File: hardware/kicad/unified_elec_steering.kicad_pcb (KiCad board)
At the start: 2 copper layers, 77.2 x 87.7 mm, 24 parts, among them J1 Conn_01x03, J10 Conn_01x04, J11 Conn_01x03, J13 Conn_01x03, J2 Conn_01x03, J3 Conn_01x05, J4 Conn_01x03, J5 Conn_01x03, J6 Conn_01x02, J7 Conn_01x04, J8 Conn_01x12, J9 Conn_01x04, U1 Arduino_Nano_v3.x, U2 D24V150F7

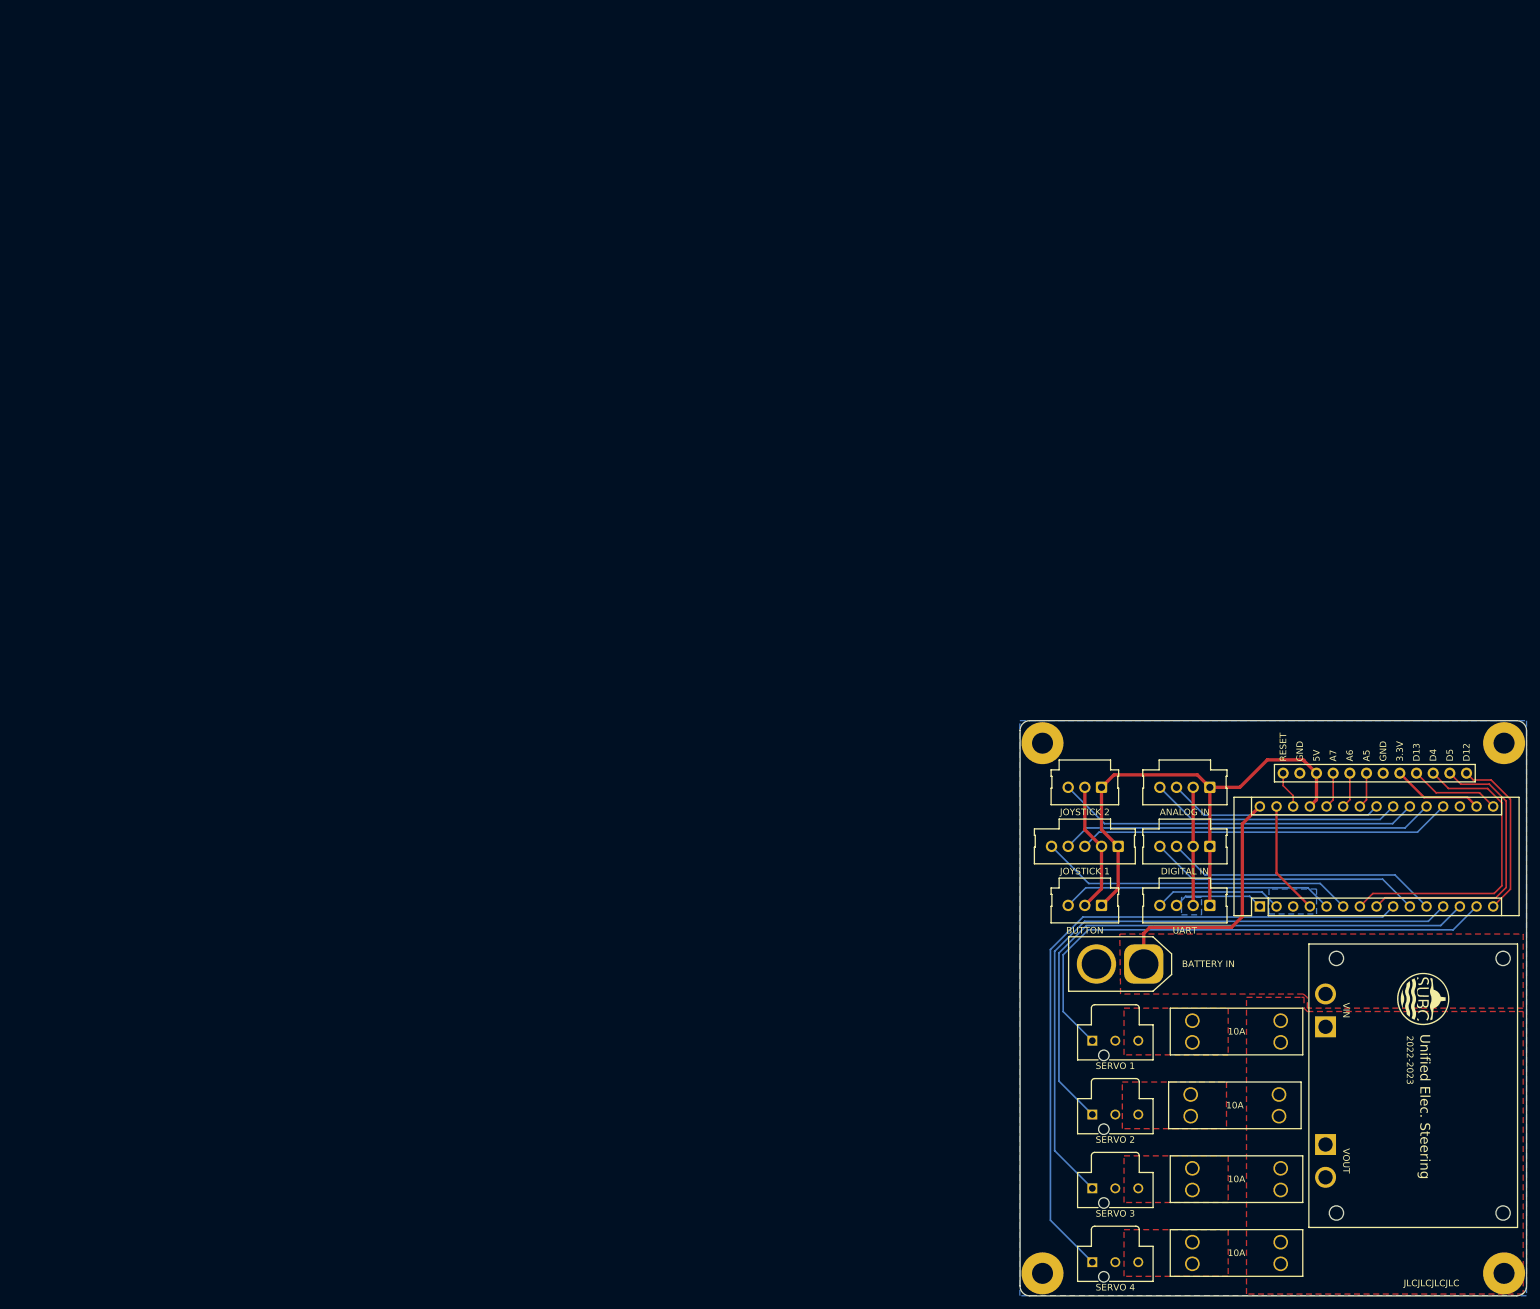
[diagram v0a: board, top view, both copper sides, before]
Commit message: Initial commit of circle PCB
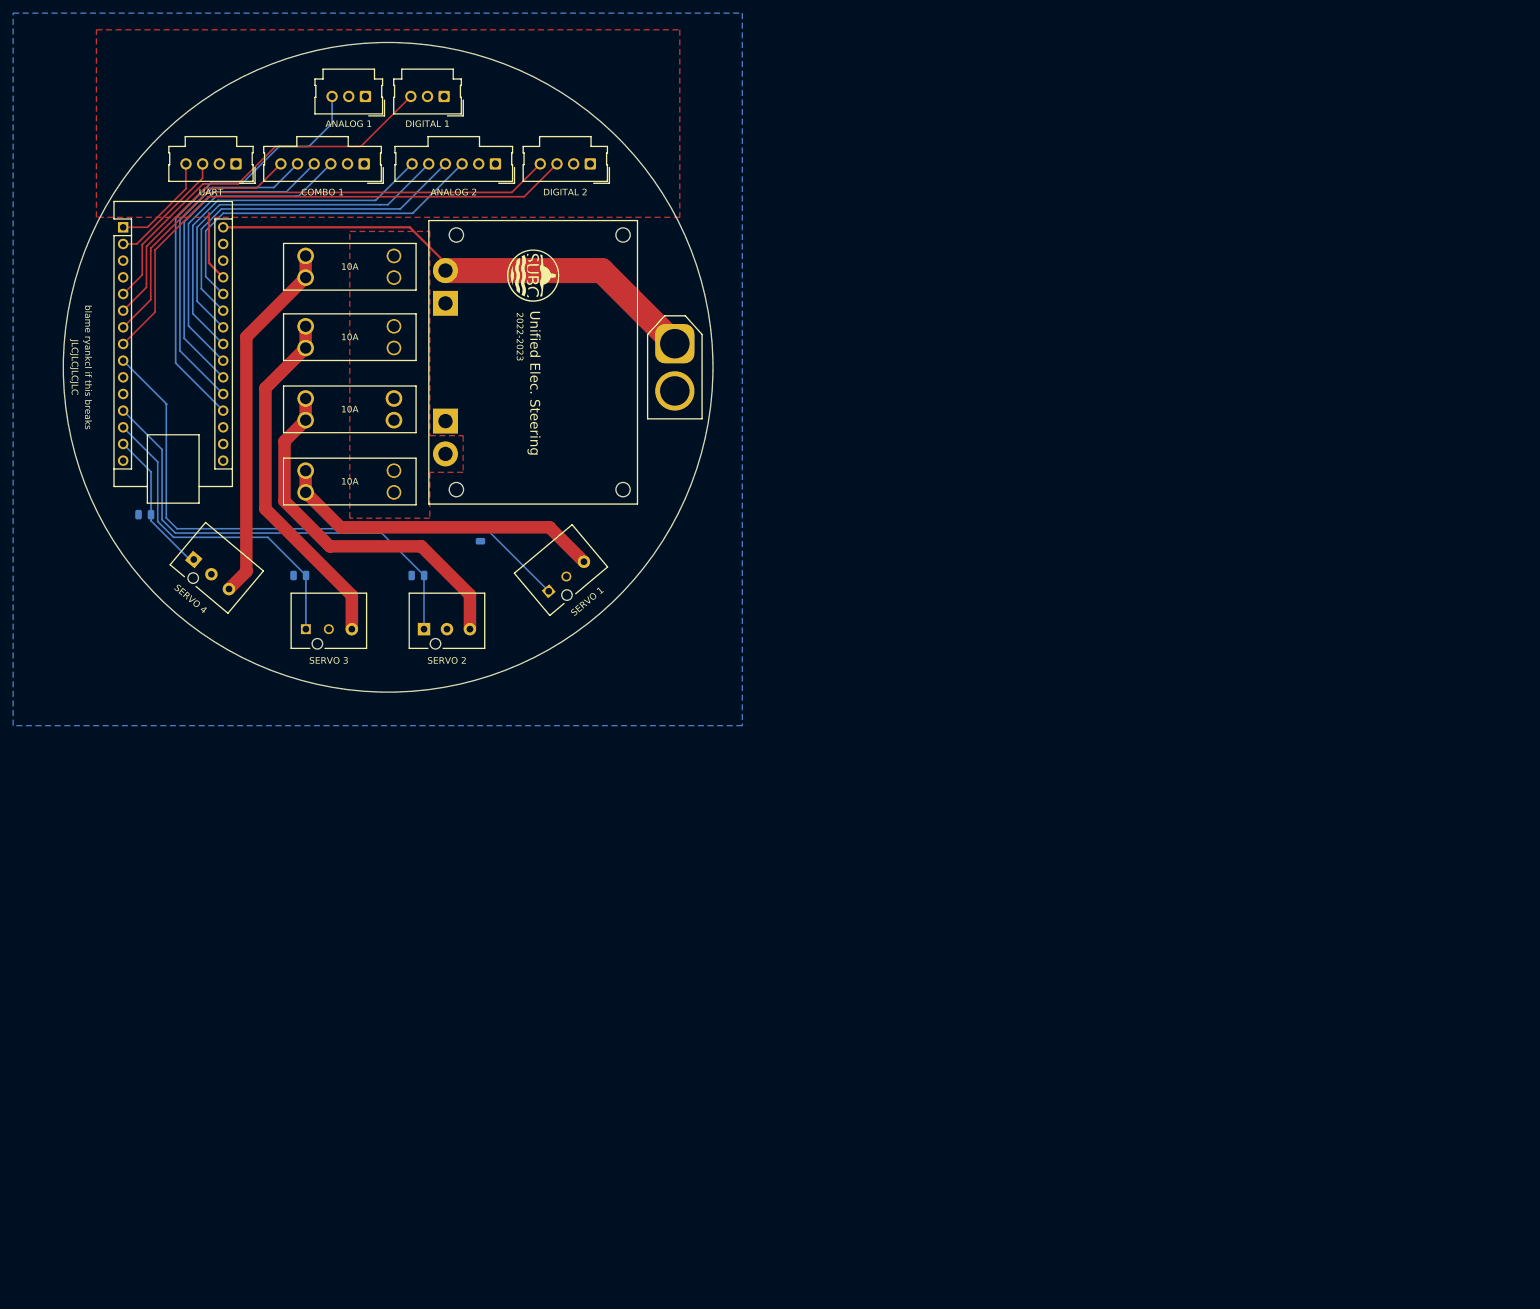
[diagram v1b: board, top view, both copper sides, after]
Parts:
- removed F5: Fuse, elec_steering:3557-2
- removed the G*** at (157.7, 96.3)
- removed the G*** at (147.6, 99.3)
- removed J1, J2: Conn_01x03, elec_steering:1722861103_ultra
- removed REF** (x4): MountingHole_3.2mm_M3_Pad, MountingHole:MountingHole_3.2mm_M3_Pad
- added C1: C_0805_2012Metric, Capacitor_SMD:C_0805_2012Metric, B.Cu at (14.1, 25.6)
- added C2: C_0805_2012Metric, Capacitor_SMD:C_0805_2012Metric, B.Cu at (4.54, 31.7)
- added C3: C_0805_2012Metric, Capacitor_SMD:C_0805_2012Metric, B.Cu at (-13.5, 31.7)
- added C4: C_0805_2012Metric, Capacitor_SMD:C_0805_2012Metric, B.Cu at (-37.1, 22.5)
- added F1: Fuse, elec_steering:3557-2, F.Cu at (-5.84, -17.0)
- added G***: LOGO, LOGO, F.Cu at (22.1, -14.0)
- added G***: LOGO, LOGO, B.Cu at (15.9, 4.37)
- added J12: Conn_01x04, Connector_Molex:Molex_SL_171971-0004_1x04_P2.54mm_Vertical, F.Cu at (30.8, -31.0)
- J10, J9: value Conn_01x04 -> Conn_01x03; footprint Connector_Molex:Molex_SL_171971-0004_1x04_P2.54mm_Vertical -> elec_steering:1722861103
- J3: value Conn_01x05 -> Conn_01x02; footprint Connector_Molex:Molex_SL_171971-0005_1x05_P2.54mm_Vertical -> Connector_AMASS:AMASS_XT60-M_1x02_P7.20mm_Vertical
- J4, J5: footprint elec_steering:1722861103_ultra -> elec_steering:1722861103
- J6: value Conn_01x02 -> Conn_01x04; footprint Connector_AMASS:AMASS_XT60-M_1x02_P7.20mm_Vertical -> Connector_Molex:Molex_SL_171971-0004_1x04_P2.54mm_Vertical
- J7: value Conn_01x04 -> Conn_01x06; footprint Connector_Molex:Molex_SL_171971-0004_1x04_P2.54mm_Vertical -> Connector_Molex:Molex_SL_171971-0006_1x06_P2.54mm_Vertical
- J8: value Conn_01x12 -> Conn_01x06; footprint Connector_PinHeader_2.54mm:PinHeader_1x12_P2.54mm_Vertical -> Connector_Molex:Molex_SL_171971-0006_1x06_P2.54mm_Vertical
- moved U1 201.8 mm to (-40.4, -21.3), turned to 0 degrees
- moved J6 184.4 mm to (-23.2, -31.0)
- moved F3 178.6 mm to (-5.84, -6.25)
- moved U2 173.6 mm to (22.1, -0.76)
- moved F4 171.9 mm to (-5.84, 15.8)
- moved J4 170.0 mm to (-29.6, 29.3), turned to -40 degrees
- moved J8 168.0 mm to (-3.65, -31.0), turned to 180 degrees
- moved F2 165.1 mm to (-5.84, 4.75)
- moved J11 158.8 mm to (8.54, -41.3)
- moved J13 153.8 mm to (-3.46, -41.3)
- moved J7 144.5 mm to (16.4, -31.0)
- moved J5 138.4 mm to (-12.5, 39.9)
- moved J9 124.2 mm to (5.47, 39.9), turned to 0 degrees
- moved J10 111.5 mm to (24.5, 34.1), turned to 40 degrees
- moved J3 99.5 mm to (43.7, 0.00), turned to -90 degrees
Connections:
- net BUTTON0 renamed D2
- F2 pad 1: Net-(J5-Pad3) -> Net-(F2-Pad1)
- F4 pad 1: Net-(J4-Pad3) -> Net-(F4-Pad1)
- J10 pad 1: +5V -> SERVO0
- J10 pad 3: TX -> Net-(F4-Pad1)
- J13 pad 3: JOY_ROLL -> A0
- J3 pad 1: +5V -> VBUS
- J4 pad 1: SERVO1 -> SERVO3
- J4 pad 3: Net-(J4-Pad3) -> Net-(F1-Pad1)
- J5 pad 1: SERVO3 -> SERVO2
- J5 pad 3: Net-(J5-Pad3) -> Net-(F3-Pad1)
- J6 pad 1: VBUS -> +5V
- J7 pad 3: A4 -> A7
- J7 pad 4: A3 -> A6
- J8 pad 1: RESET -> +5V
- J8 pad 3: +5V -> A3
- J8 pad 4: A7 -> A2
- J8 pad 5: A6 -> A1
- J8 pad 6: A5 -> D3
- J9 pad 1: +5V -> SERVO1
- J9 pad 3: D8 -> Net-(F2-Pad1)
- U1 pad 19: JOY_PITCH -> A0
- U1 pad 20: JOY_YAW -> A1
- U1 pad 21: JOY_ROLL -> A2
- U1 pad 6: BUTTON1 -> D3
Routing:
- net +5V: track 80.5 -> 10.7 mm
- net A0: track 0.00 -> 66.2 mm
- net SERVO3: track 81.0 -> 22.4 mm
- net JOY_PITCH: track 57.1 -> 0.00 mm
- net JOY_YAW: track 57.1 -> 0.00 mm
- net Net-(F2-Pad1): track 0.00 -> 56.4 mm
- net Net-(F1-Pad1): track 0.00 -> 55.6 mm
- net JOY_ROLL: track 55.5 -> 0.00 mm
- net GND: track 55.4 -> 0.00 mm
- net Net-(F3-Pad1): track 0.00 -> 54.1 mm
- net A5: track 5.49 -> 56.2 mm
- net A1: track 0.00 -> 50.7 mm
- net Net-(F4-Pad1): track 0.00 -> 50.1 mm
- net A6: track 5.49 -> 55.1 mm
- net A2: track 0.00 -> 49.6 mm
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- added copper zone on F.Cu, net +5V
- removed copper zone on F.Cu, net Net-(F3-Pad1)
- removed copper zone on F.Cu, net Net-(J2-Pad3)
- removed copper zone on F.Cu, net Net-(J4-Pad3)
- removed copper zone on F.Cu, net Net-(J5-Pad3)
- removed copper zone on F.Cu, net VBUS
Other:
- board size 77.2 x 87.7 mm -> 99 x 99 mm
- board text added: "ANALOG 1"
- board text added: "ANALOG 2"
- board text added: "COMBO 1"
- board text added: "DIGITAL 1"
- board text added: "DIGITAL 2"
- board text added: "blame ryankcl if this breaks"
- board text removed: "3.3V"
- board text removed: "5V"
- board text removed: "A5"
- board text removed: "A6"
- board text removed: "A7"
- board text removed: "ANALOG IN"
- board text removed: "BATTERY IN"
- board text removed: "BUTTON"
- board text removed: "Conn_01x12"
- board text removed: "D12"
- board text removed: "D13"
- board text removed: "D4"
- board text removed: "D5"
- board text removed: "DIGITAL IN"
- board text removed: "GND"
- board text removed: "JOYSTICK 1"
- board text removed: "JOYSTICK 2"
- board text removed: "RESET"
- board text removed: "VIN"
- board text removed: "VOUT"
